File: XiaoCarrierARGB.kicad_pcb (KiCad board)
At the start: 2 copper layers, 76.4 x 50.8 mm, 24 parts, among them J1 V_{IN}^{10-24V}, J2 Conn_01x08, J3 Conn_01x01, J4 Conn_01x08, J5 Conn_01x01, J6 Conn_01x06, U1 TLV75733PDBV, U2 TPP362083-T6TR, U3 XIAO-ESP32-C6-DIP, U4 74LVC1T45W6-7, U5 74LVC1T45W6-7, U6 74LVC1T45W6-7

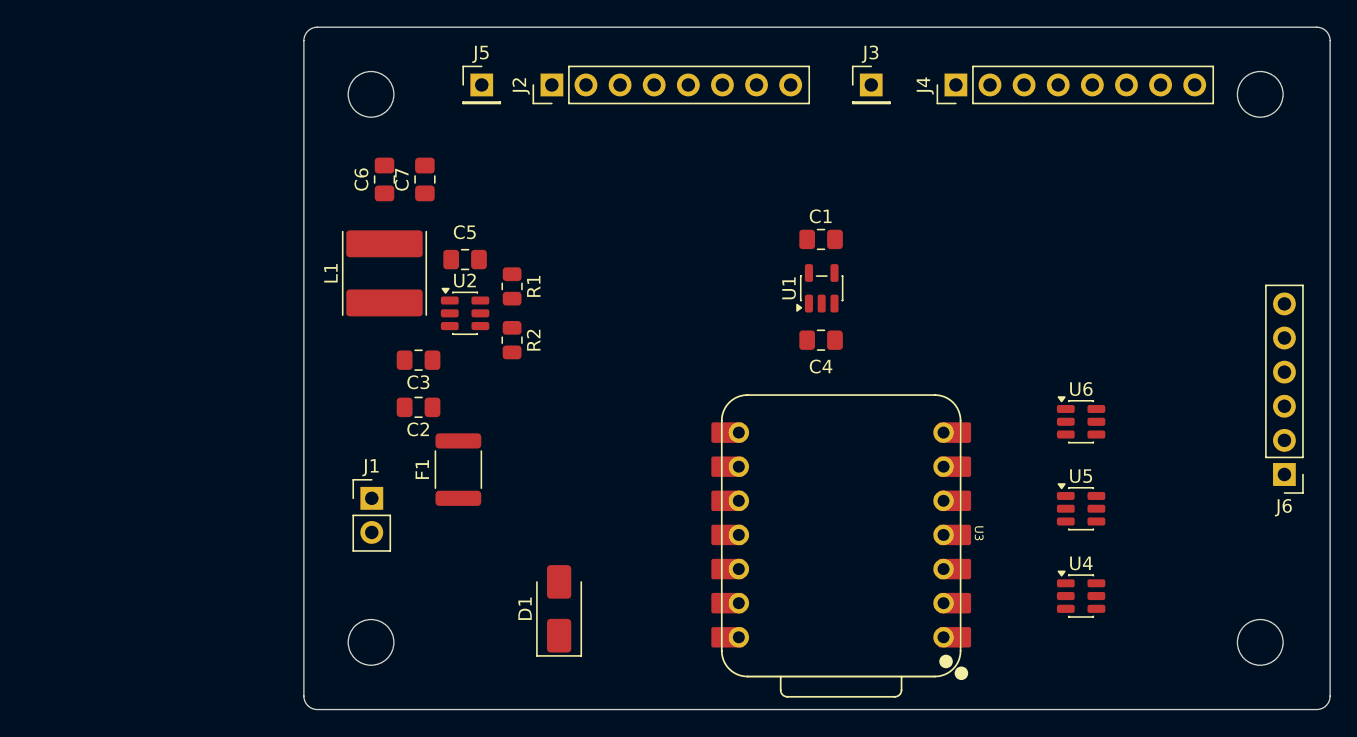
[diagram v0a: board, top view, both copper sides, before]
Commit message: adjusted prelim layout
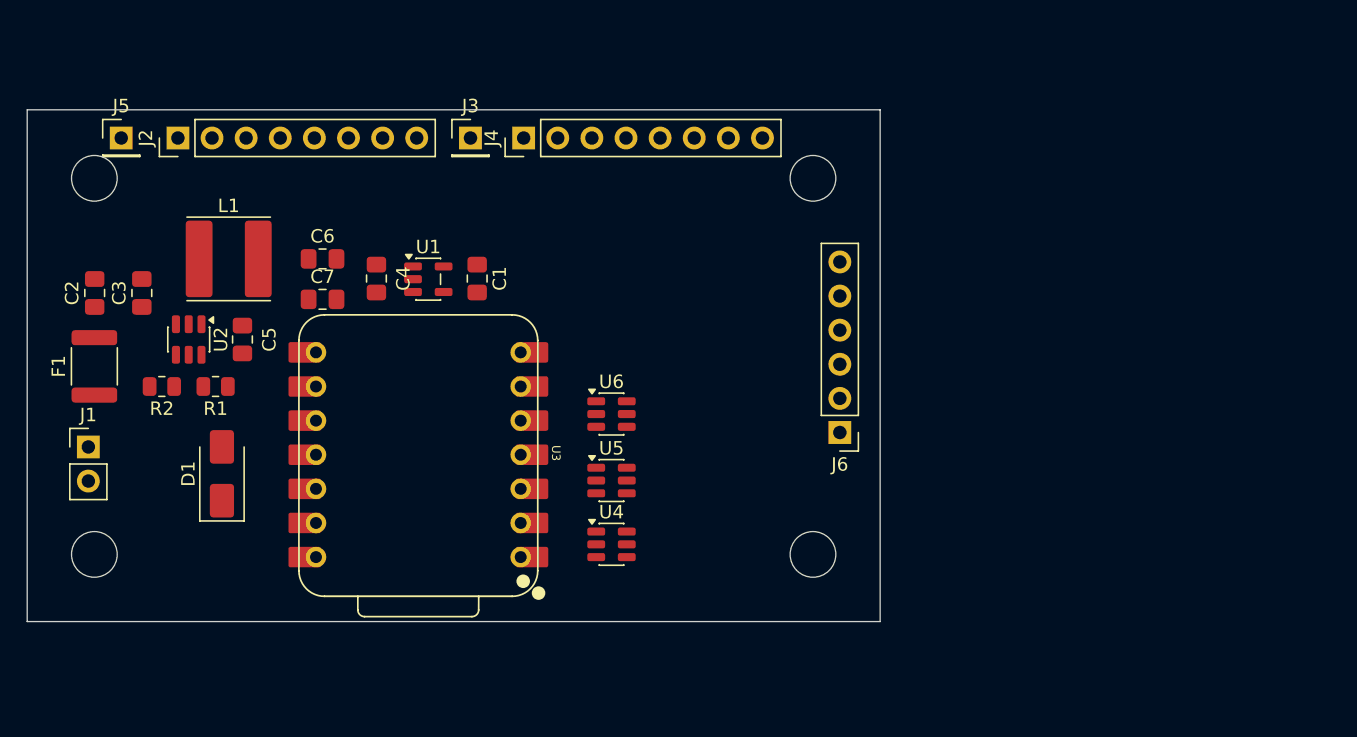
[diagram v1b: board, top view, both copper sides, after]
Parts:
- moved U4 35.2 mm to (131.8, 113.3)
- moved U5 35.0 mm to (131.8, 108.5)
- moved U6 35.0 mm to (131.8, 103.6)
- moved C4 33.4 mm to (114.2, 93.5), turned to 90 degrees
- moved J6 33.2 mm to (148.8, 105.0)
- moved J4 32.4 mm to (125.2, 83.0)
- moved U3 32.0 mm to (117.4, 106.6)
- moved J3 30.1 mm to (121.2, 83.0)
- moved U1 29.3 mm to (118.1, 93.6), turned to 0 degrees
- moved F1 28.2 mm to (93.2, 100.0)
- moved J2 28.1 mm to (99.5, 83.0)
- moved J5 27.1 mm to (95.2, 83.0)
- moved D1 27.0 mm to (102.8, 108.0)
- moved R2 26.3 mm to (98.3, 101.5), turned to 180 degrees
- moved C1 25.8 mm to (121.8, 93.5), turned to -90 degrees
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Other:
- board size 76.4 x 50.8 mm -> 63.5 x 38.1 mm
